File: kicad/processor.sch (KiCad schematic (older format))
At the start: 22 parts, among them J1 USB-C, U1 LP5907MFX-3.3, U2 SRV05-4, U3 STM32F072C8Tx

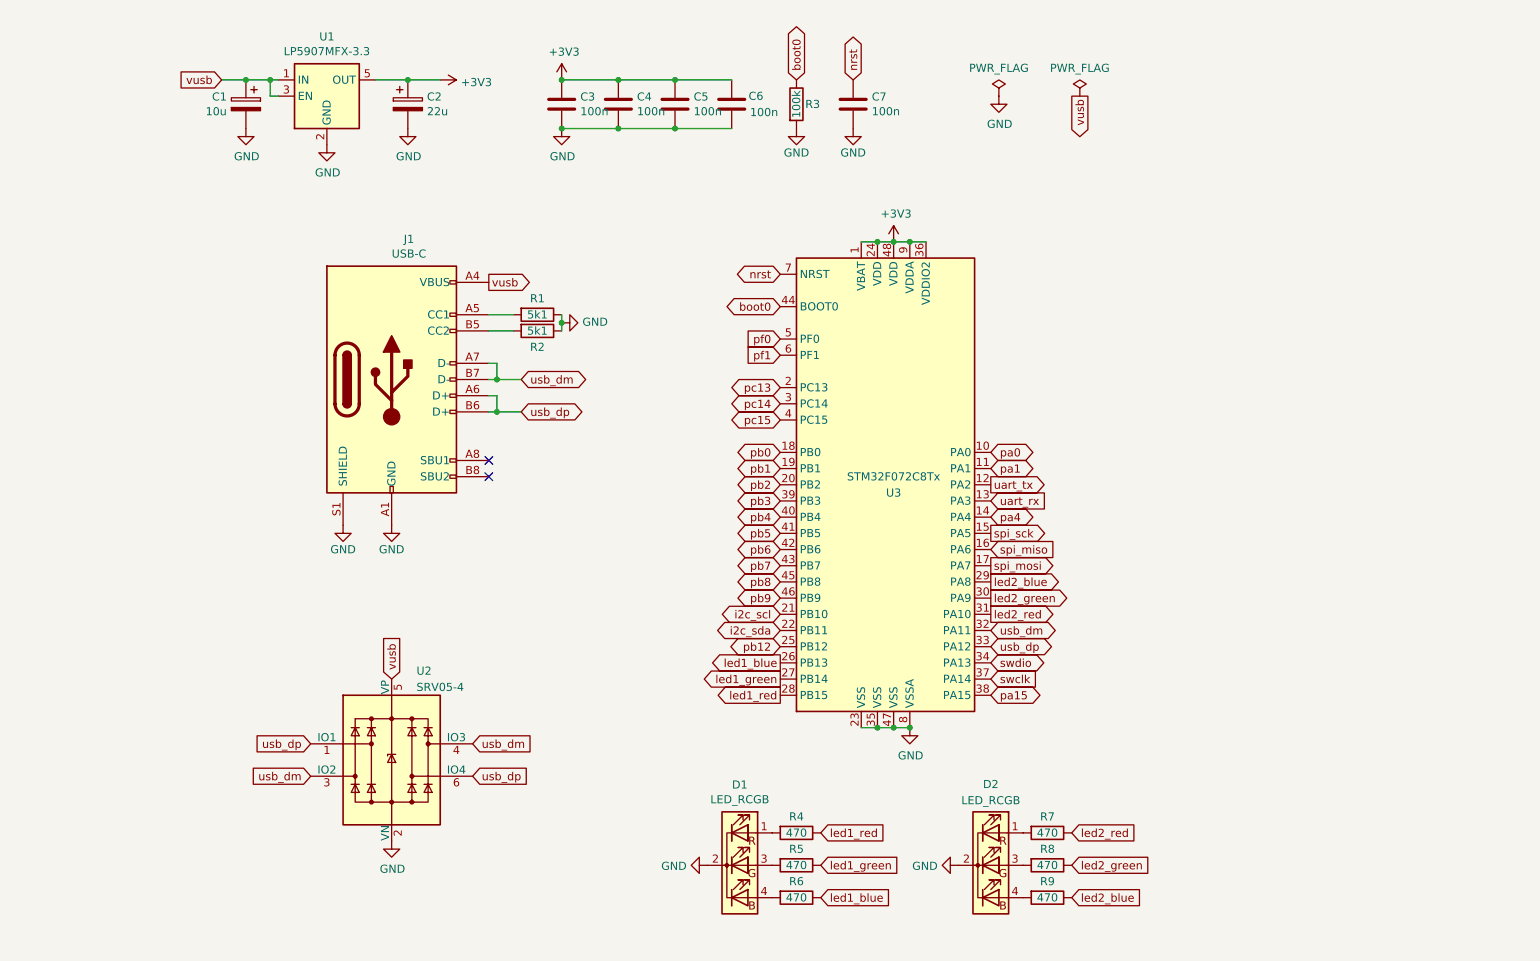
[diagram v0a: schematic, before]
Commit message: Krieger_v2.00
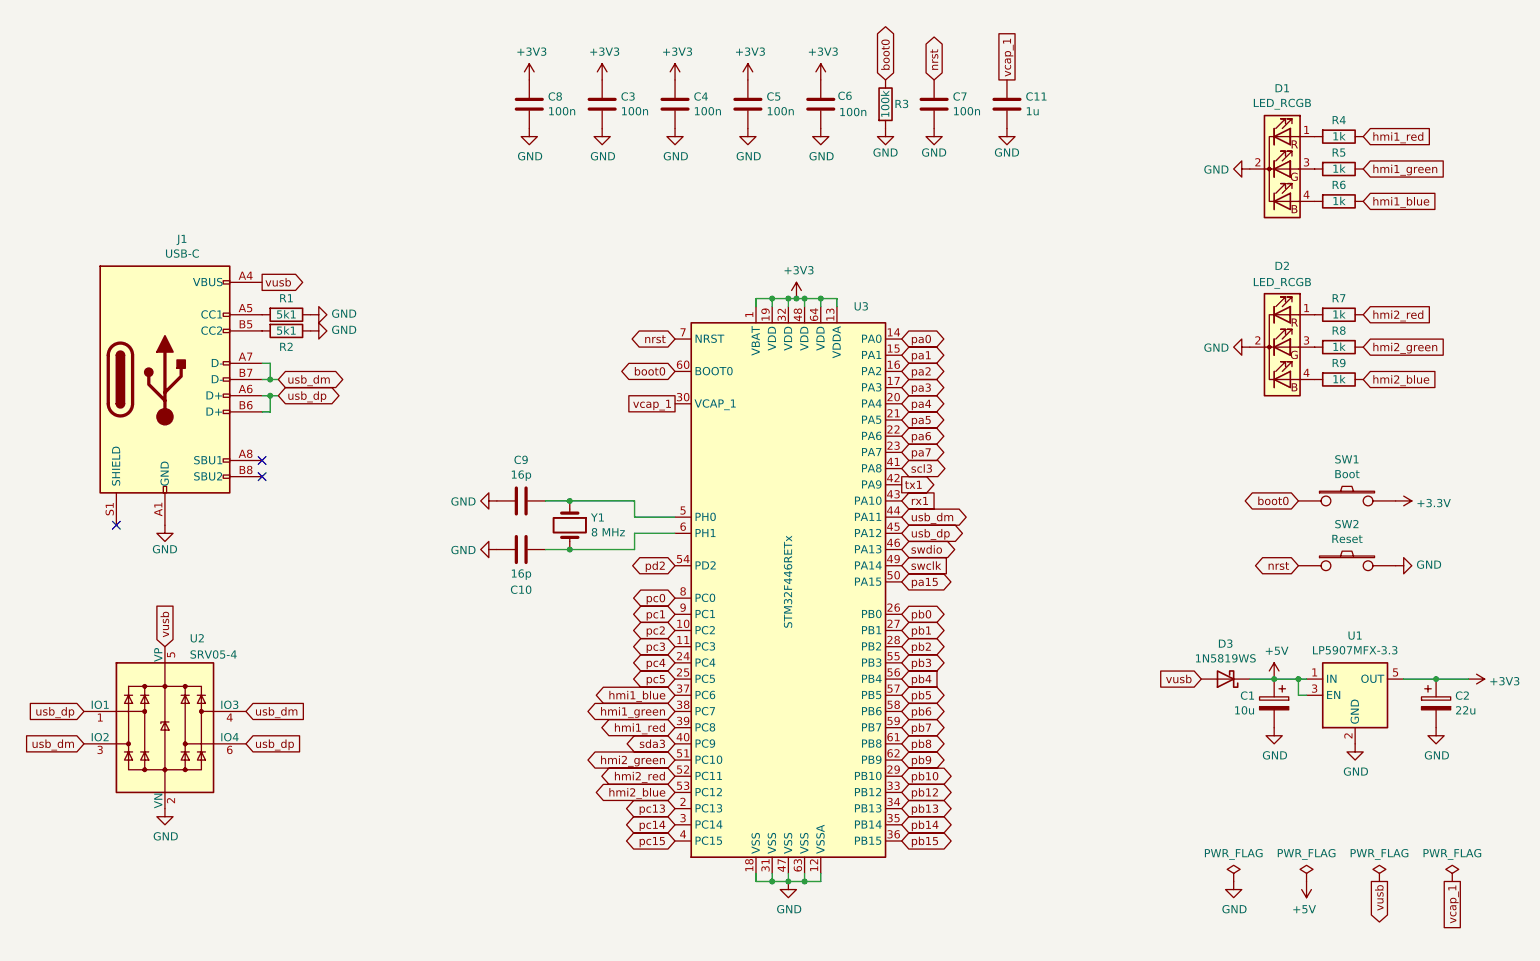
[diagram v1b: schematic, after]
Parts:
- removed U3: STM32F072C8Tx, Package_QFP:LQFP-48_7x7mm_P0.5mm, symbol MCU_ST_STM32F0:STM32F072C8Tx
- added C10, C9: 16p, Capacitor_SMD:C_0603_1608Metric, symbol Device:C
- added C11: 1u, Capacitor_SMD:C_0603_1608Metric, symbol Device:C
- added C8: 100n, Capacitor_SMD:C_0603_1608Metric, symbol Device:C
- added D3: 1N5819WS, Diode_SMD:D_SOD-323_HandSoldering, symbol Device:D_Schottky
- added SW1: Boot, krieger:TACT-SWITCH, symbol krieger:TACT-SWITCH
- added SW2: Reset, krieger:TACT-SWITCH, symbol krieger:TACT-SWITCH
- added U3: STM32F446RETx, Package_QFP:LQFP-64_10x10mm_P0.5mm, symbol MCU_ST_STM32F4:STM32F446RETx
- added Y1: 8 MHz, Crystal:Crystal_SMD_5032-2Pin_5.0x3.2mm, symbol Device:Crystal
- R4, R5, R6, R7, R8, R9: value 470 -> 1k
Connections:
- net +3V3: now also C8.1, SW1.2, U3.1 (VBAT), U3.13 (VDDA), U3.19 (VDD), U3.32 (VDD), U3.48 (VDD), U3.64 (VDD)
- net GND: now also C10.2, C11.2, C8.2, C9.2, SW2.2, U3.12 (VSSA), U3.18 (VSS), U3.31 (VSS), U3.47 (VSS), U3.63 (VSS); no longer J1.S1 (SHIELD)
- net boot0: now also SW1.1, U3.60 (BOOT0)
- net nrst: now also SW2.1, U3.7 (NRST)
- net pa0: now also U3.14 (PA0)
- net pa1: now also U3.15 (PA1)
- net pa15: now also U3.50 (PA15)
- net pa4: now also U3.20 (PA4)
- net pb0: now also U3.26 (PB0)
- net pb1: now also U3.27 (PB1)
- net pb12: now also U3.33 (PB12)
- net pb2: now also U3.28 (PB2)
- net pb3: now also U3.55 (PB3)
- net pb4: now also U3.56 (PB4)
- net pb5: now also U3.57 (PB5)
- net pb6: now also U3.58 (PB6)
- net pb7: now also U3.59 (PB7)
- net pb8: now also U3.61 (PB8)
- net pb9: now also U3.62 (PB9)
- net pc13: now also U3.2 (PC13)
- net pc14: now also U3.3 (PC14)
- net pc15: now also U3.4 (PC15)
- net swclk: now also U3.49 (PA14)
- net swdio: now also U3.46 (PA13)
- net usb_dm: now also U3.44 (PA11)
- net usb_dp: now also U3.45 (PA12)
- net vusb: now also D3.2 (A); no longer C1.1, U1.1 (IN), U1.3 (EN)
- net led1_blue renamed hmi1_blue
- net hmi1_blue: now also U3.37 (PC6)
- net led1_green renamed hmi1_green
- net hmi1_green: now also U3.38 (PC7)
- net led1_red renamed hmi1_red
- net hmi1_red: now also U3.39 (PC8)
- net led2_blue renamed hmi2_blue
- net hmi2_blue: now also U3.53 (PC12)
- net led2_green renamed hmi2_green
- net hmi2_green: now also U3.51 (PC10)
- net led2_red renamed hmi2_red
- net hmi2_red: now also U3.52 (PC11)
- new net: C9.1, U3.5 (PH0), Y1.1
- new net: C10.1, U3.6 (PH1), Y1.2
- new net +5V: C1.1, D3.1 (K), U1.1 (IN), U1.3 (EN)
- new net pa2: U3.16 (PA2)
- new net pa3: U3.17 (PA3)
- new net pa5: U3.21 (PA5)
- new net pa6: U3.22 (PA6)
- new net pa7: U3.23 (PA7)
- new net pb10: U3.29 (PB10)
- new net pb13: U3.34 (PB13)
- new net pb14: U3.35 (PB14)
- new net pb15: U3.36 (PB15)
- new net pc0: U3.8 (PC0)
- new net pc1: U3.9 (PC1)
- new net pc2: U3.10 (PC2)
- new net pc3: U3.11 (PC3)
- new net pc4: U3.24 (PC4)
- new net pc5: U3.25 (PC5)
- new net pd2: U3.54 (PD2)
- new net rx1: U3.43 (PA10)
- new net scl3: U3.41 (PA8)
- new net sda3: U3.40 (PC9)
- new net tx1: U3.42 (PA9)
- new net vcap_1: C11.1, U3.30 (VCAP_1)
- no-connect marks 2 -> 3
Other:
- moved on the sheet: C1, C2, C3, C4, C5, C6, C7, D1, D2, J1, R1, R2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

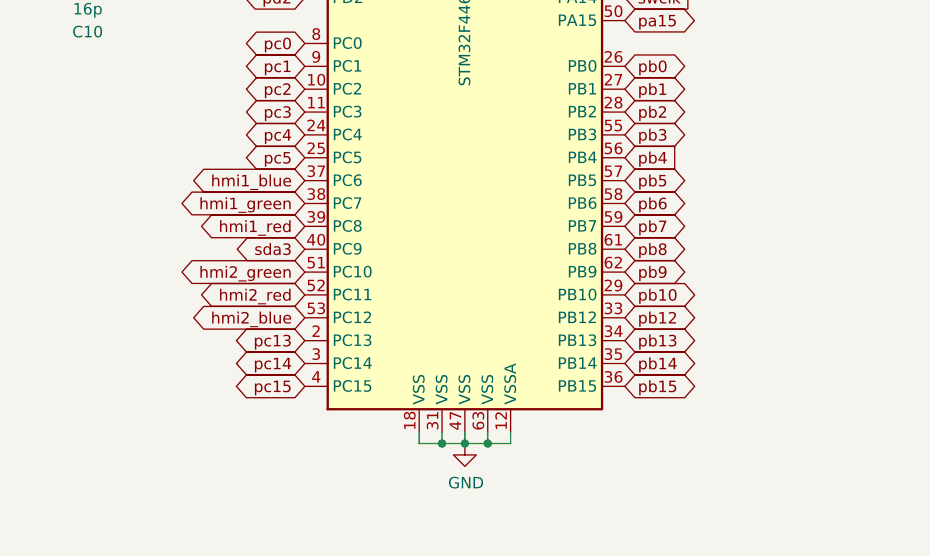
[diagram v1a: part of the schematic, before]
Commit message: Krieger v2.00
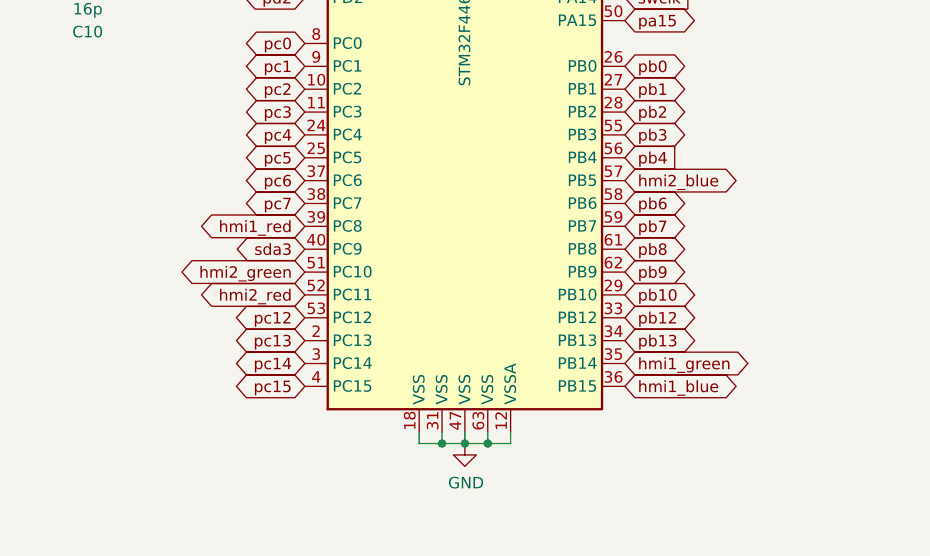
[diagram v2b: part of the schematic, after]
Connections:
- net pb14 is gone; now on net hmi1_green: U3.35 (PB14)
- net pb15 is gone; now on net hmi1_blue: U3.36 (PB15)
- net pb5 is gone; now on net hmi2_blue: U3.57 (PB5)
- net hmi1_blue: no longer U3.37 (PC6)
- net hmi1_green: no longer U3.38 (PC7)
- net hmi2_blue: no longer U3.53 (PC12)
- new net pc12: U3.53 (PC12)
- new net pc6: U3.37 (PC6)
- new net pc7: U3.38 (PC7)
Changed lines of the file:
@@
 Sheet 2 3
 Title "Krieger"
-Date "2021-05-24"
+Date "2021-06-05"
 Rev "v2.0"
 Comp "www.2-0.dk"
@@
 Text GLabel 6800 2850 2    50   BiDi ~ 0
 pa1
-Text GLabel 5400 5550 0    50   BiDi ~ 0
+Text GLabel 6800 4950 2    50   BiDi ~ 0
 hmi2_blue
 Text GLabel 5400 4150 0    50   BiDi ~ 0
@@
 Text GLabel 6800 4250 2    50   BiDi ~ 0
 pa15
-Text GLabel 6800 4950 2    50   BiDi ~ 0
-pb5
+Text GLabel 5400 5550 0    50   BiDi ~ 0
+pc12
 Text GLabel 6800 5050 2    50   BiDi ~ 0
 pb6
@@
 Text GLabel 6800 5650 2    50   BiDi ~ 0
 pb13
-Text GLabel 6800 5750 2    50   BiDi ~ 0
-pb14
-Text GLabel 6800 5850 2    50   BiDi ~ 0
-pb15
 $Comp
 L MCU_ST_STM32F4:STM32F446RETx U3
@@
 	1    0    0    -1
 $EndComp
-Text GLabel 5400 4950 0    50   BiDi ~ 0
+Text GLabel 6800 5850 2    50   BiDi ~ 0
 hmi1_blue
-Text GLabel 5400 5050 0    50   BiDi ~ 0
+Text GLabel 6800 5750 2    50   BiDi ~ 0
 hmi1_green
 Text GLabel 5400 5150 0    50   BiDi ~ 0
@@
 	0    1    1    0
 $EndComp
+Text GLabel 5400 4950 0    50   BiDi ~ 0
+pc6
+Text GLabel 5400 5050 0    50   BiDi ~ 0
+pc7
 $EndSCHEMATC
